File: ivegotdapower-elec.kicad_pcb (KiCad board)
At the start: 2 copper layers, 70 x 92 mm, 69 parts, among them J1 Conn_Debug, J10 Conn_+3.3V, J11 Conn_bau, J12 CAN_conn, J13 CAN_conn, J2 Conn_batt, J3 Conn_alim, J4 Conn_TSMR, J5 Conn_POW2, J6 Conn_POW1, J7 Conn_RPi, J8 Conn_+5V, Q1 IRFR5305, Q2 IRFR5305, Q3 BSS138, Q4 MMBT2907A, Q5 MMBT2907A, Q6 MMBT2907A, Q7 MMBT2907A, U1 TCAN332, U10 LD1117S33TR_SOT223, U11 LM358, U6 ACS711xLCTR-12AB, U7 STM32F303K8Tx, U8 LD1117S50TR_SOT223

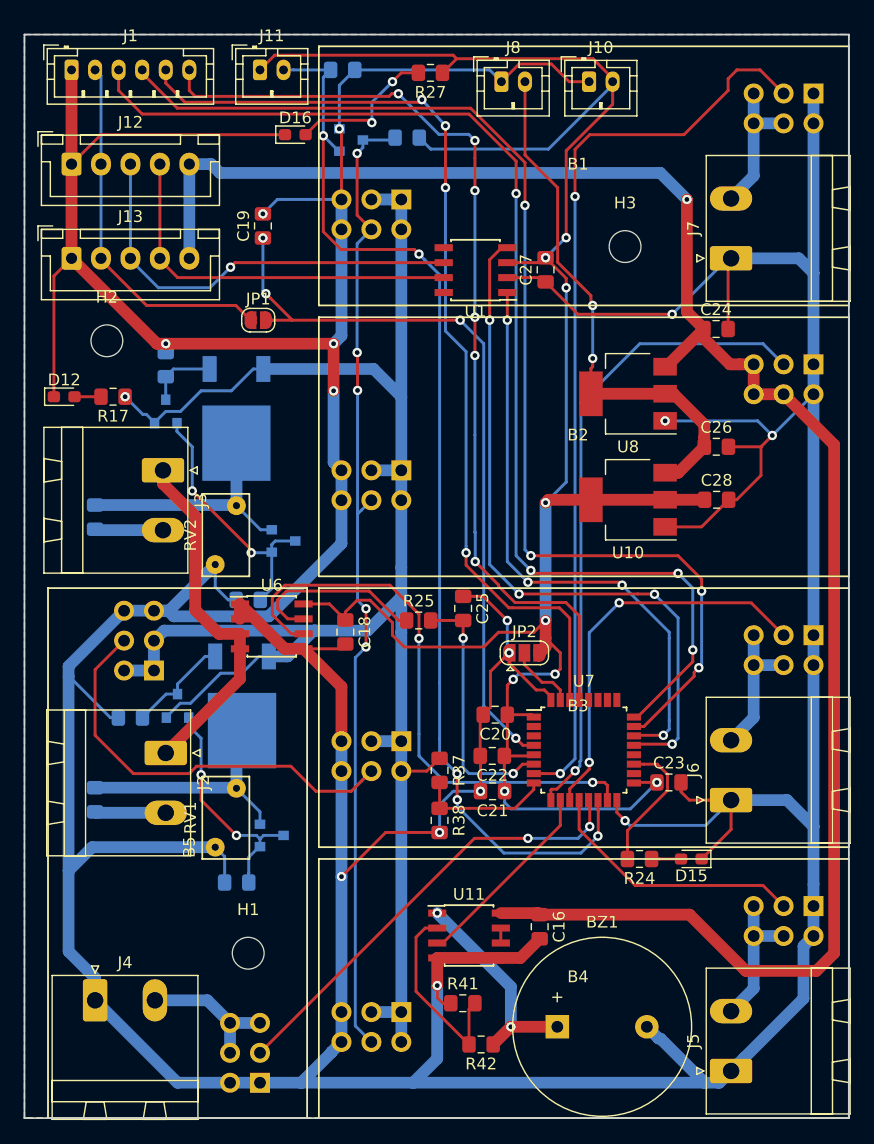
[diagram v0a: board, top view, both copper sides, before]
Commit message: update board_fille
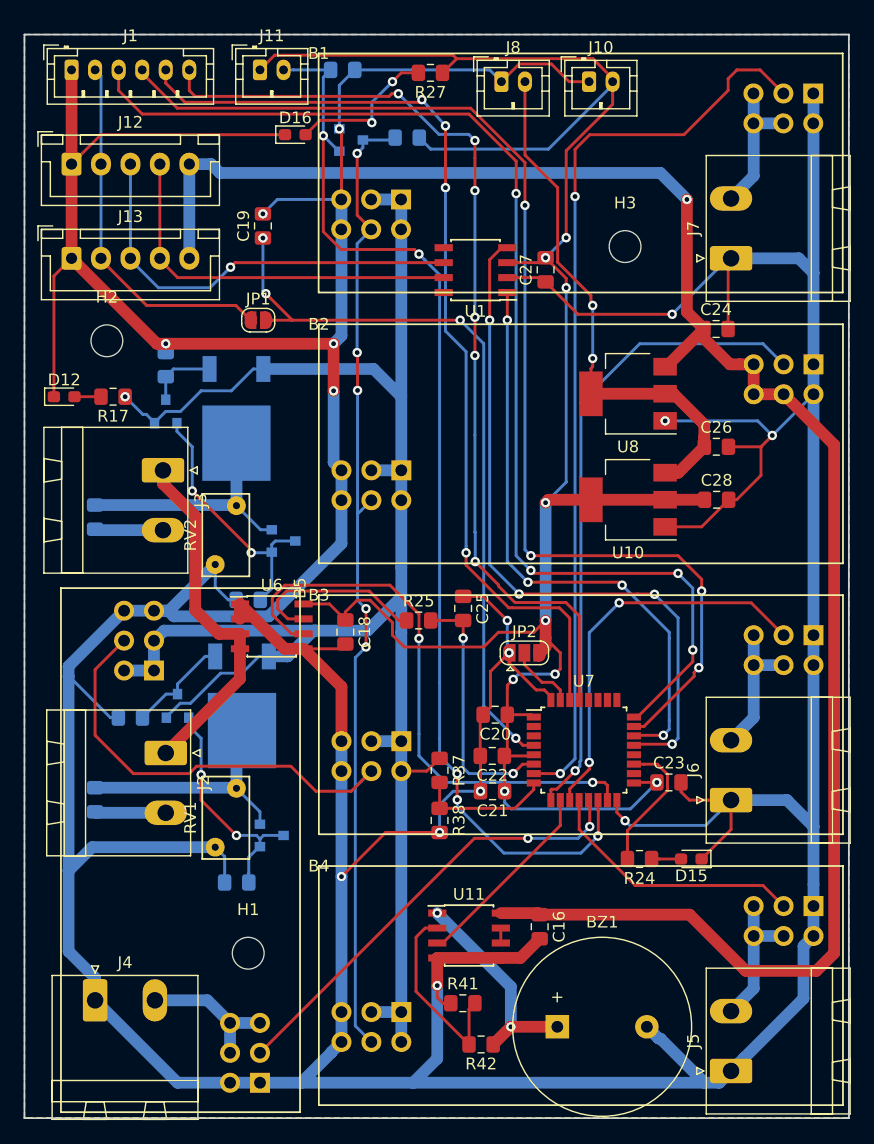
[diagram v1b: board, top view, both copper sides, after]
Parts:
- moved B1 23.9 mm to (101.0, 100.6)
- moved B2 23.9 mm to (101.0, 123.6)
- moved B3 23.9 mm to (101.0, 146.6)
- moved B4 23.9 mm to (101.0, 169.6)
- moved B5 23.9 mm to (99.4, 146.0)
